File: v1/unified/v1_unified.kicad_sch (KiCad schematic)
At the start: 81 parts, among them U1 XIAO-RP2040-SMD, U2 CY8CMBR3116, U3 CY8CMBR3116

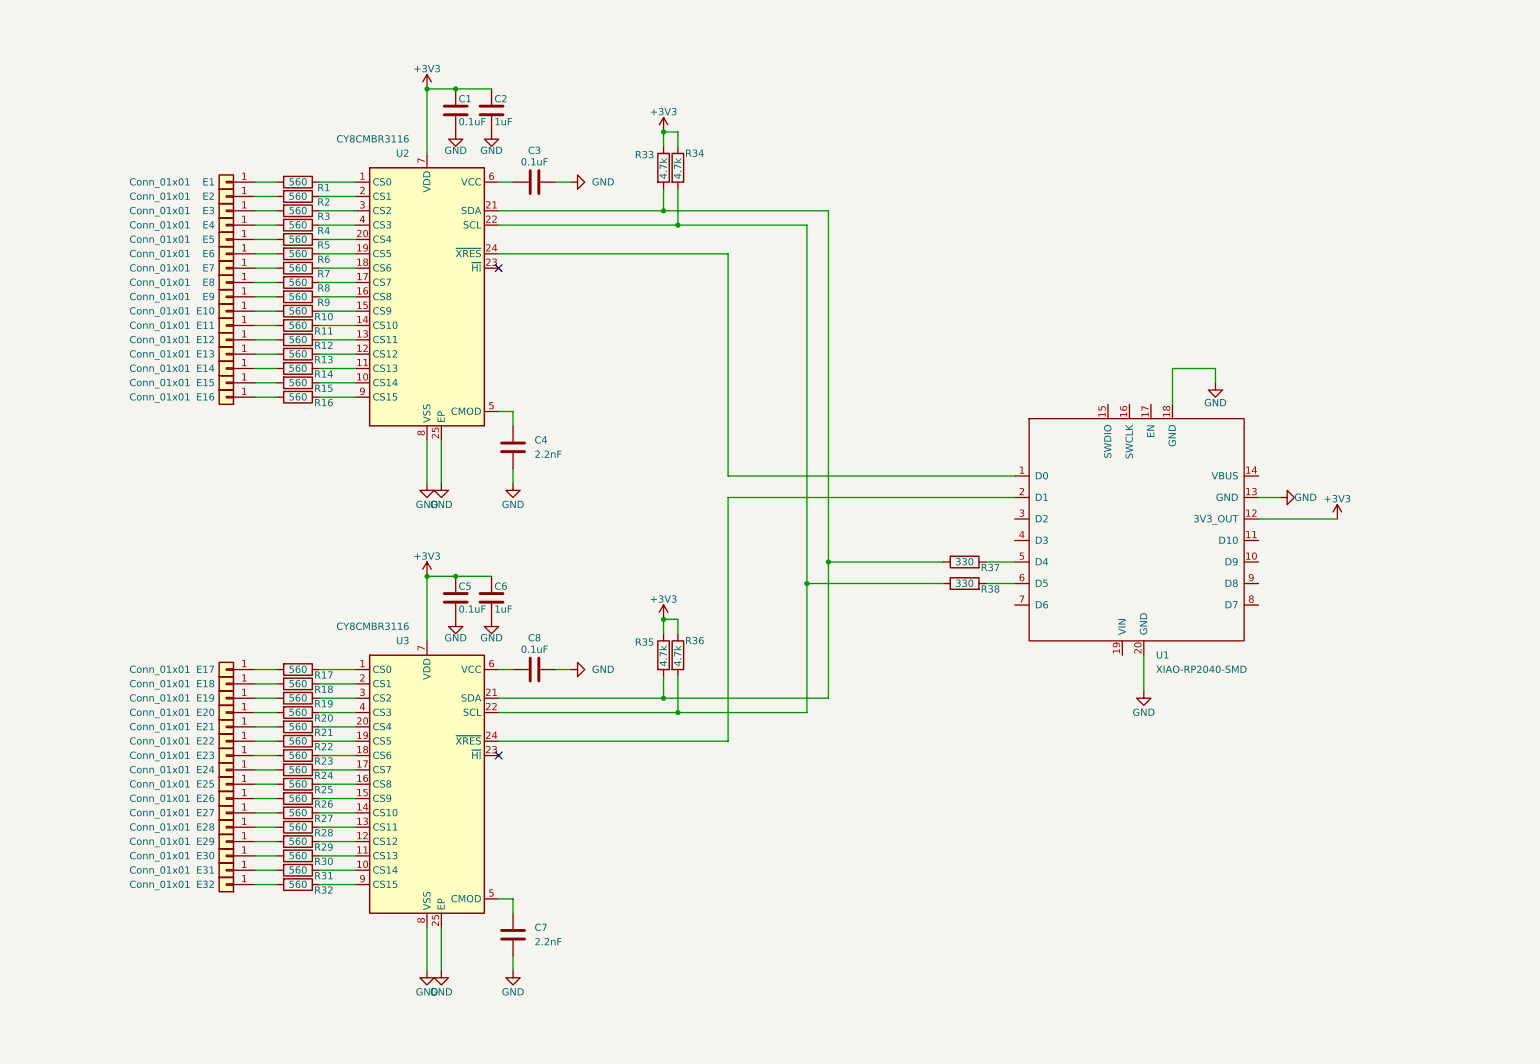
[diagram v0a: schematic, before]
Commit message: fix
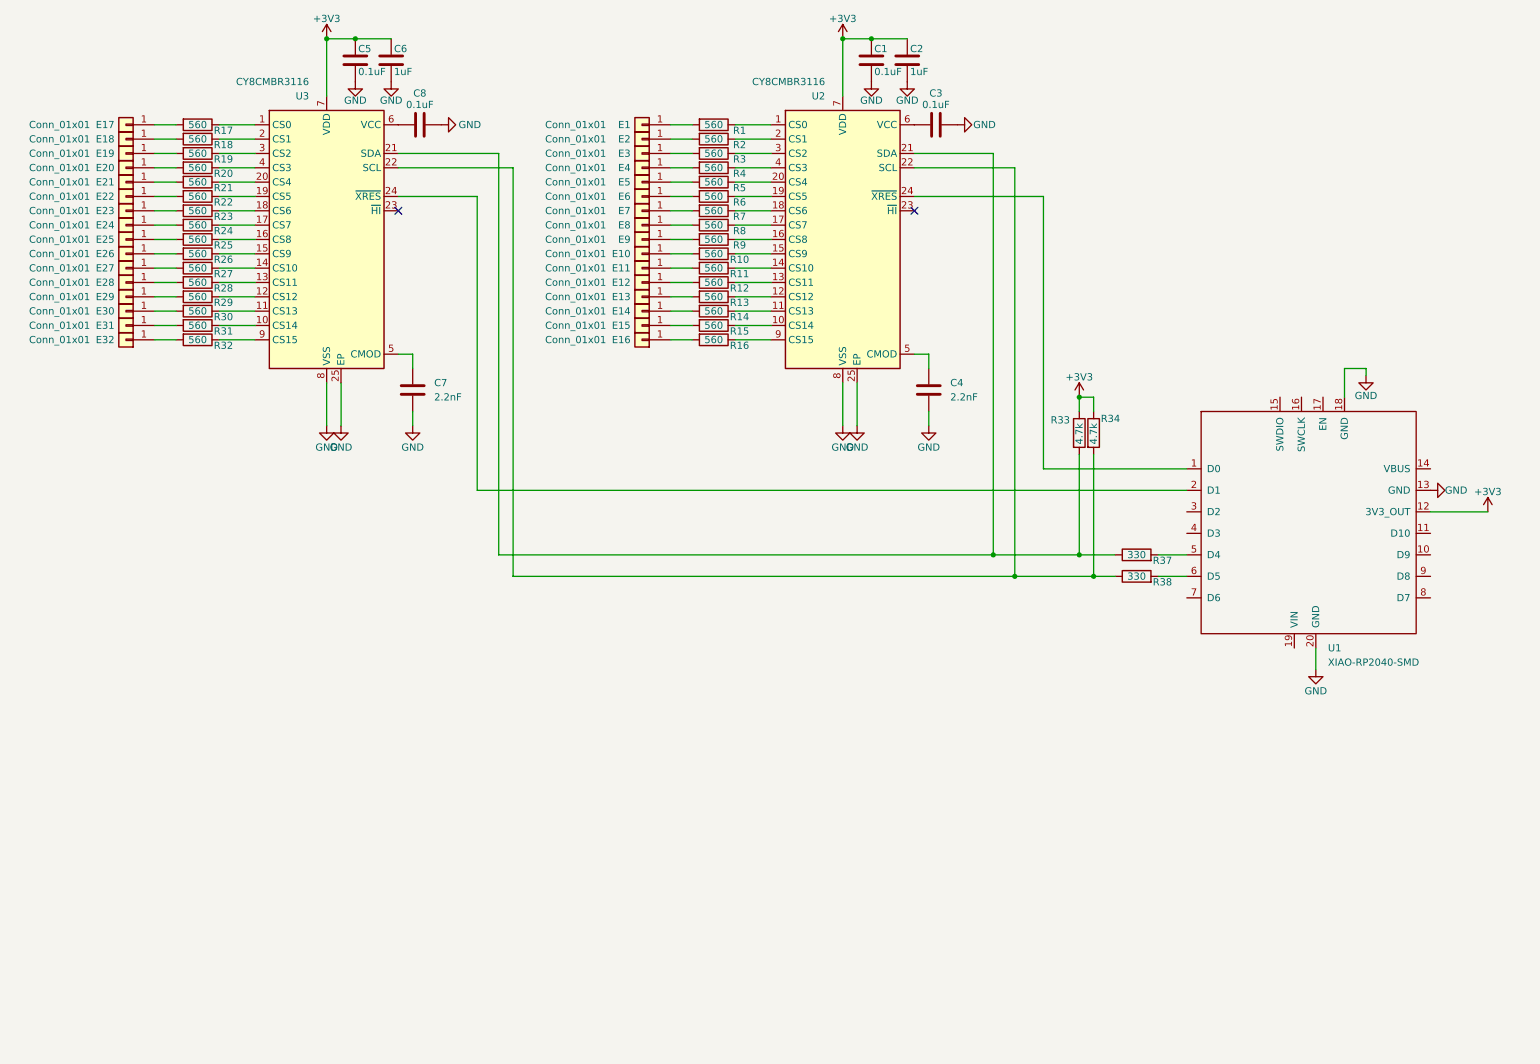
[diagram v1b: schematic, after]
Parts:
- removed R35, R36: 4.7k, symbol Device:R
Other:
- moved on the sheet: C1, C2, C3, C4, C5, C6, C7, C8, E1, E10, E11, E12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

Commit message: feat: add LED
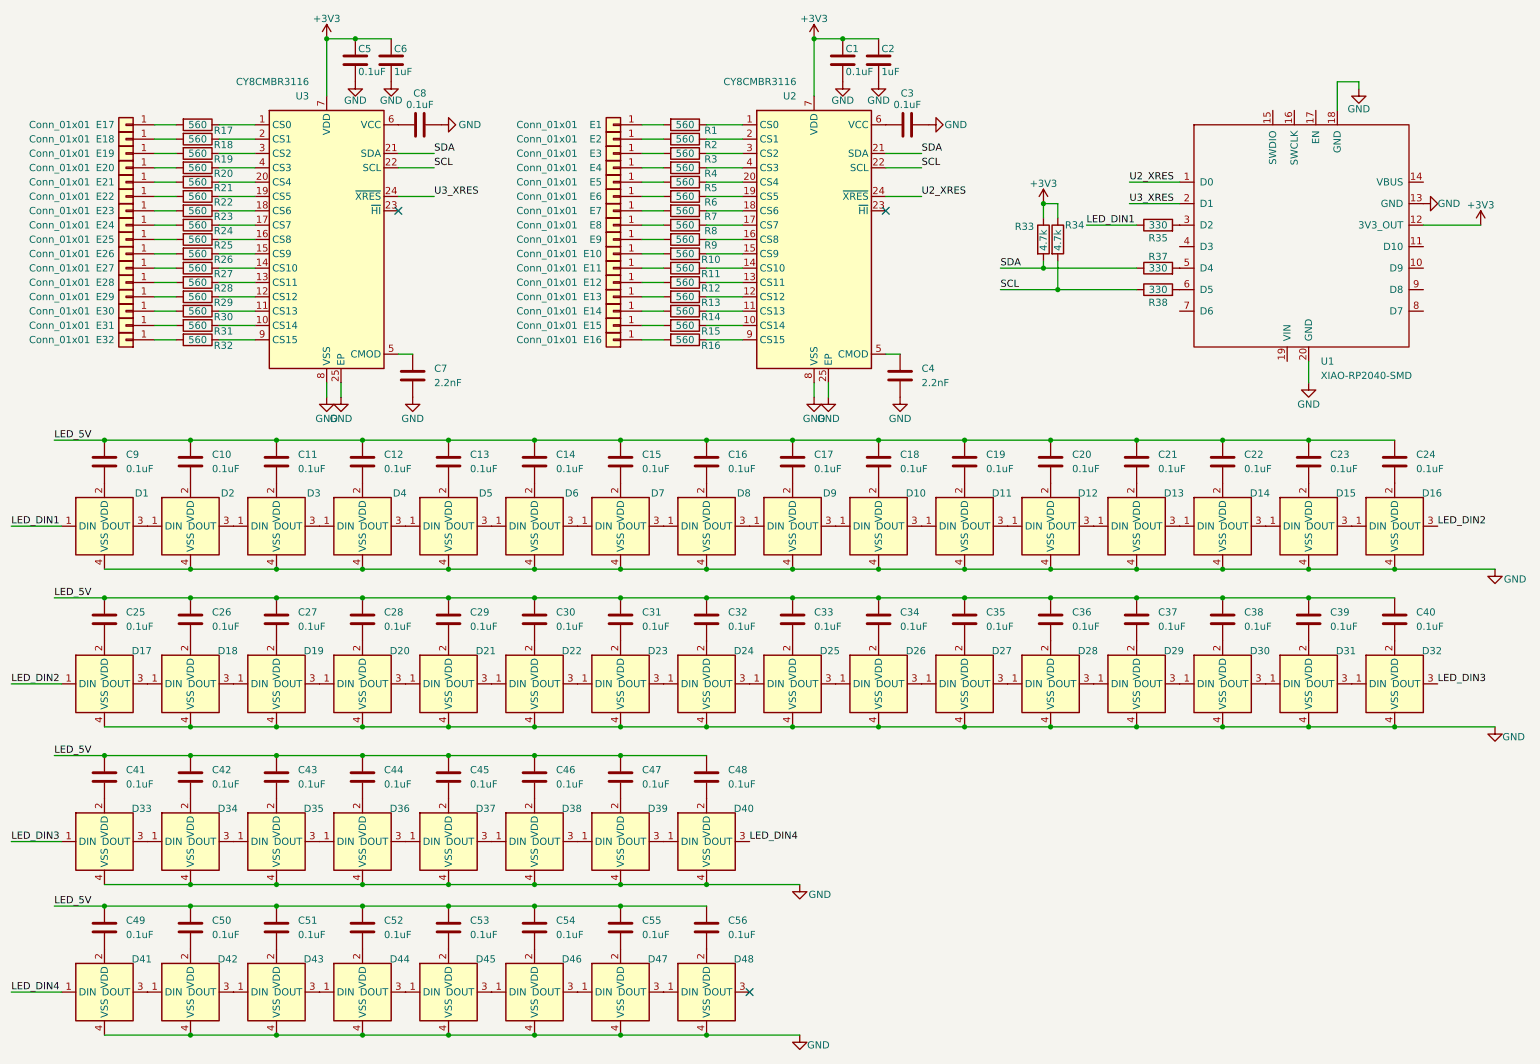
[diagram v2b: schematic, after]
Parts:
- added C10, C11, C12, C13, C14, C15, C16, C17, C18, C19, C20, C21, C22, C23, C24, C25, C26, C27, C28, C29, C30, C31, C32, C33, C34, C35, C36, C37, C38, C39, C40, C41, C42, C43, C44, C45, C46, C47, C48, C49, C50, C51, C52, C53, C54, C55, C56, C9: 0.1uF, symbol Device:C
- added D1, D10, D11, D12, D13, D14, D15, D16, D17, D18, D19, D2, D20, D21, D22, D23, D24, D25, D26, D27, D28, D29, D3, D30, D31, D32, D33, D34, D35, D36, D37, D38, D39, D4, D40, D41, D42, D43, D44, D45, D46, D47, D48, D5, D6, D7, D8, D9: WS2812B-4020-V6, v1_common:WS2812B-4020-V6, symbol v1_common:WS2812B-4020-V6
- added R35: 330, symbol Device:R
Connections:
- net GND: now also D1.4 (VSS), D10.4 (VSS), D11.4 (VSS), D12.4 (VSS), D13.4 (VSS), D14.4 (VSS), D15.4 (VSS), D16.4 (VSS), D17.4 (VSS), D18.4 (VSS), D19.4 (VSS), D2.4 (VSS), D20.4 (VSS), D21.4 (VSS), D22.4 (VSS), D23.4 (VSS), D24.4 (VSS), D25.4 (VSS), D26.4 (VSS), D27.4 (VSS), D28.4 (VSS), D29.4 (VSS), D3.4 (VSS), D30.4 (VSS), D31.4 (VSS), D32.4 (VSS), D33.4 (VSS), D34.4 (VSS), D35.4 (VSS), D36.4 (VSS), D37.4 (VSS), D38.4 (VSS), D39.4 (VSS), D4.4 (VSS), D40.4 (VSS), D41.4 (VSS), D42.4 (VSS), D43.4 (VSS), D44.4 (VSS), D45.4 (VSS), D46.4 (VSS), D47.4 (VSS), D48.4 (VSS), D5.4 (VSS), D6.4 (VSS), D7.4 (VSS), D8.4 (VSS), D9.4 (VSS)
- net SCL: now reaches R34.2, R38.1, U2.22 (SCL), U3.22 (SCL)
- net SDA: now reaches R33.2, R37.1, U2.21 (SDA), U3.21 (SDA)
- net U3_XRES: now reaches U1.2 (D1), U3.24 (~{XRES})
- net U2_XRES: now reaches U1.1 (D0), U2.24 (~{XRES})
- net at U1.3 (D2): now also R35.2
- new net: C30.2, D22.2 (VDD)
- new net: C33.2, D25.2 (VDD)
- new net: D42.3 (DOUT), D43.1 (DIN)
- new net: C51.2, D43.2 (VDD)
- new net: D43.3 (DOUT), D44.1 (DIN)
- new net: D13.3 (DOUT), D14.1 (DIN)
- new net: C22.2, D14.2 (VDD)
- new net: D14.3 (DOUT), D15.1 (DIN)
- new net: D5.3 (DOUT), D6.1 (DIN)
- new net: C14.2, D6.2 (VDD)
- new net: D6.3 (DOUT), D7.1 (DIN)
- new net: D10.3 (DOUT), D11.1 (DIN)
- new net: C19.2, D11.2 (VDD)
- new net: D11.3 (DOUT), D12.1 (DIN)
- new net: C25.2, D17.2 (VDD)
- new net: C41.2, D33.2 (VDD)
- new net: C17.2, D9.2 (VDD)
- new net: D10.1 (DIN), D9.3 (DOUT)
- new net: C18.2, D10.2 (VDD)
- new net: D21.3 (DOUT), D22.1 (DIN)
- new net: D22.3 (DOUT), D23.1 (DIN)
- new net: C45.2, D37.2 (VDD)
- new net: C46.2, D38.2 (VDD)
- new net: C21.2, D13.2 (VDD)
- new net: C12.2, D4.2 (VDD)
- new net: D33.3 (DOUT), D34.1 (DIN)
- new net: C42.2, D34.2 (VDD)
- new net: D34.3 (DOUT), D35.1 (DIN)
- new net: D41.3 (DOUT), D42.1 (DIN)
- new net: C50.2, D42.2 (VDD)
- new net: C23.2, D15.2 (VDD)
- new net: C37.2, D29.2 (VDD)
- new net: C32.2, D24.2 (VDD)
- new net: D17.3 (DOUT), D18.1 (DIN)
- new net: C20.2, D12.2 (VDD)
- new net: C11.2, D3.2 (VDD)
- new net: C43.2, D35.2 (VDD)
- new net: D35.3 (DOUT), D36.1 (DIN)
- new net: C48.2, D40.2 (VDD)
- new net: D19.3 (DOUT), D20.1 (DIN)
- new net: C28.2, D20.2 (VDD)
- new net: D20.3 (DOUT), D21.1 (DIN)
- new net: C44.2, D36.2 (VDD)
- new net: D36.3 (DOUT), D37.1 (DIN)
- new net: C53.2, D45.2 (VDD)
- new net: C36.2, D28.2 (VDD)
- new net: C38.2, D30.2 (VDD)
- new net: D37.3 (DOUT), D38.1 (DIN)
- new net: C55.2, D47.2 (VDD)
- new net: D1.3 (DOUT), D2.1 (DIN)
- new net: C10.2, D2.2 (VDD)
- new net: D2.3 (DOUT), D3.1 (DIN)
- new net: C31.2, D23.2 (VDD)
- new net: D15.3 (DOUT), D16.1 (DIN)
- new net: D45.3 (DOUT), D46.1 (DIN)
- new net: C54.2, D46.2 (VDD)
- new net: D46.3 (DOUT), D47.1 (DIN)
- new net: D8.3 (DOUT), D9.1 (DIN)
- new net: C49.2, D41.2 (VDD)
- new net: D7.3 (DOUT), D8.1 (DIN)
- new net: C16.2, D8.2 (VDD)
- new net: C39.2, D31.2 (VDD)
- new net: C35.2, D27.2 (VDD)
- new net: D31.3 (DOUT), D32.1 (DIN)
- new net: C40.2, D32.2 (VDD)
- new net: D47.3 (DOUT), D48.1 (DIN)
- new net: C56.2, D48.2 (VDD)
- new net: D27.3 (DOUT), D28.1 (DIN)
- new net: D28.3 (DOUT), D29.1 (DIN)
- new net: D3.3 (DOUT), D4.1 (DIN)
- new net: D4.3 (DOUT), D5.1 (DIN)
- new net: D12.3 (DOUT), D13.1 (DIN)
- new net: D38.3 (DOUT), D39.1 (DIN)
- new net: C47.2, D39.2 (VDD)
- new net: D39.3 (DOUT), D40.1 (DIN)
- new net: C15.2, D7.2 (VDD)
- new net: D23.3 (DOUT), D24.1 (DIN)
- new net: C29.2, D21.2 (VDD)
- new net: D25.3 (DOUT), D26.1 (DIN)
- new net: C34.2, D26.2 (VDD)
- new net: D26.3 (DOUT), D27.1 (DIN)
- new net: C9.2, D1.2 (VDD)
- new net: C24.2, D16.2 (VDD)
- new net: D30.3 (DOUT), D31.1 (DIN)
- new net: D29.3 (DOUT), D30.1 (DIN)
- new net: C27.2, D19.2 (VDD)
- new net: C13.2, D5.2 (VDD)
- new net: D44.3 (DOUT), D45.1 (DIN)
- new net: C26.2, D18.2 (VDD)
- new net: D18.3 (DOUT), D19.1 (DIN)
- new net: D24.3 (DOUT), D25.1 (DIN)
- new net: C52.2, D44.2 (VDD)
- new net LED_5V: C10.1, C11.1, C12.1, C13.1, C14.1, C15.1, C16.1, C17.1, C18.1, C19.1, C20.1, C21.1, C22.1, C23.1, C24.1, C25.1, C26.1, C27.1, C28.1, C29.1, C30.1, C31.1, C32.1, C33.1, C34.1, C35.1, C36.1, C37.1, C38.1, C39.1, C40.1, C41.1, C42.1, C43.1, C44.1, C45.1, C46.1, C47.1, C48.1, C49.1, C50.1, C51.1, C52.1, C53.1, C54.1, C55.1, C56.1, C9.1
- new net LED_DIN1: D1.1 (DIN), R35.1
- new net LED_DIN2: D16.3 (DOUT), D17.1 (DIN)
- new net LED_DIN3: D32.3 (DOUT), D33.1 (DIN)
- new net LED_DIN4: D40.3 (DOUT), D41.1 (DIN)
- no-connect marks 2 -> 3
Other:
- moved on the sheet: C1, C2, C3, C4, C7, E1, E10, E11, E12, E13, E14, E15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

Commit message: feat: add LED
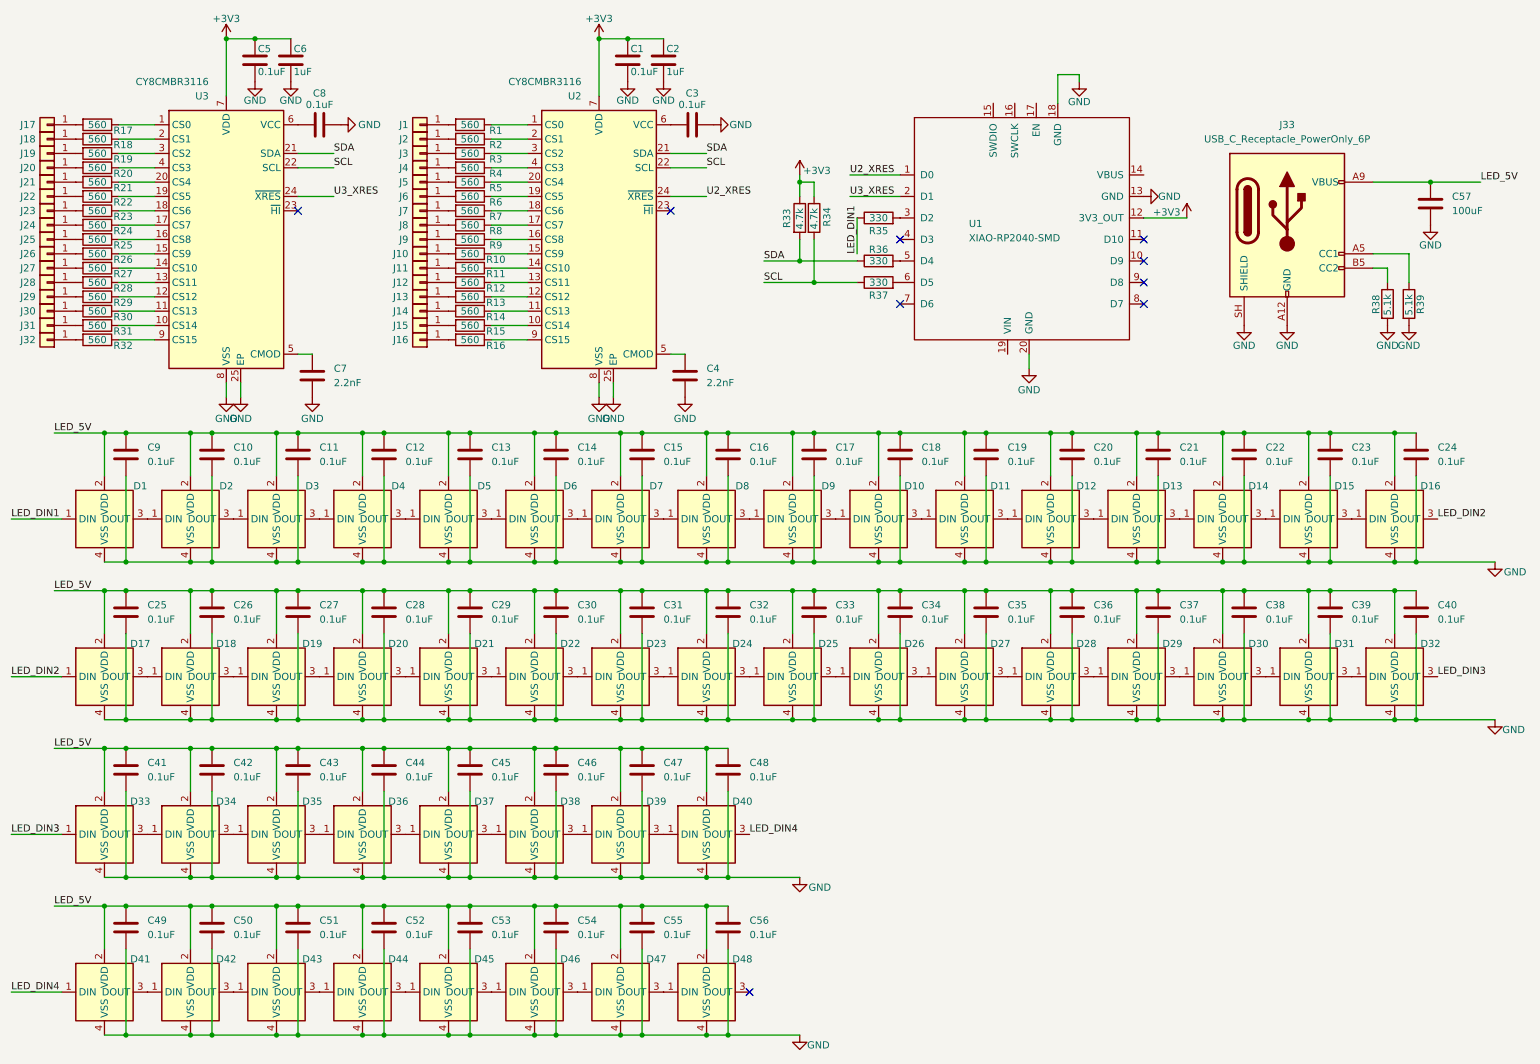
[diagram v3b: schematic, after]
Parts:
- added C57: 100uF, symbol Device:C
- added J33: USB_C_Receptacle_PowerOnly_6P, symbol Connector:USB_C_Receptacle_PowerOnly_6P
- added R38, R39: 5.1k, symbol Device:R
- renumbered E1 to J1, E10 to J10, E11 to J11, E12 to J12, E13 to J13, E14 to J14, E15 to J15, E16 to J16, E17 to J17, E18 to J18, E19 to J19, E2 to J2, E20 to J20, E21 to J21, E22 to J22, E23 to J23, E24 to J24, E25 to J25, E26 to J26, E27 to J27, E28 to J28, E29 to J29, E3 to J3, E30 to J30, E31 to J31, E32 to J32, E4 to J4, E5 to J5, E6 to J6, E7 to J7, E8 to J8, E9 to J9, R37 to R36, R38 to R37
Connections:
- net GND: now also C10.2, C11.2, C12.2, C13.2, C14.2, C15.2, C16.2, C17.2, C18.2, C19.2, C20.2, C21.2, C22.2, C23.2, C24.2, C25.2, C26.2, C27.2, C28.2, C29.2, C30.2, C31.2, C32.2, C33.2, C34.2, C35.2, C36.2, C37.2, C38.2, C39.2, C40.2, C41.2, C42.2, C43.2, C44.2, C45.2, C46.2, C47.2, C48.2, C49.2, C50.2, C51.2, C52.2, C53.2, C54.2, C55.2, C56.2, C9.2, C57.2, J33.A12 (GND), J33.B12 (GND), J33.SH (SHIELD), R38.2, R39.2
- net LED_5V: now also D1.2 (VDD), D10.2 (VDD), D11.2 (VDD), D12.2 (VDD), D13.2 (VDD), D14.2 (VDD), D15.2 (VDD), D16.2 (VDD), D17.2 (VDD), D18.2 (VDD), D19.2 (VDD), D2.2 (VDD), D20.2 (VDD), D21.2 (VDD), D22.2 (VDD), D23.2 (VDD), D24.2 (VDD), D25.2 (VDD), D26.2 (VDD), D27.2 (VDD), D28.2 (VDD), D29.2 (VDD), D3.2 (VDD), D30.2 (VDD), D31.2 (VDD), D32.2 (VDD), D33.2 (VDD), D34.2 (VDD), D35.2 (VDD), D36.2 (VDD), D37.2 (VDD), D38.2 (VDD), D39.2 (VDD), D4.2 (VDD), D40.2 (VDD), D41.2 (VDD), D42.2 (VDD), D43.2 (VDD), D44.2 (VDD), D45.2 (VDD), D46.2 (VDD), D47.2 (VDD), D48.2 (VDD), D5.2 (VDD), D6.2 (VDD), D7.2 (VDD), D8.2 (VDD), D9.2 (VDD), C57.1, J33.A9 (VBUS), J33.B9 (VBUS)
- new net: J33.A5 (CC1), R39.1
- new net: J33.B5 (CC2), R38.1
- no-connect marks 3 -> 9
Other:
- moved on the sheet: C1, C2, C27, C28, C29, C3, C30, C31, C32, C33, C34, C35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
